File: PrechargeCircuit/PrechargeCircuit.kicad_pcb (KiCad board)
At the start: 2 copper layers, 102.6 x 57.8 mm, 53 parts, among them J1 430450428, J2 430450428, J4 436500228, U1 TEA 1-0505E, U2 AMC1351DWVR, U3 AMC1351DWVR, U6 OP284EPZ

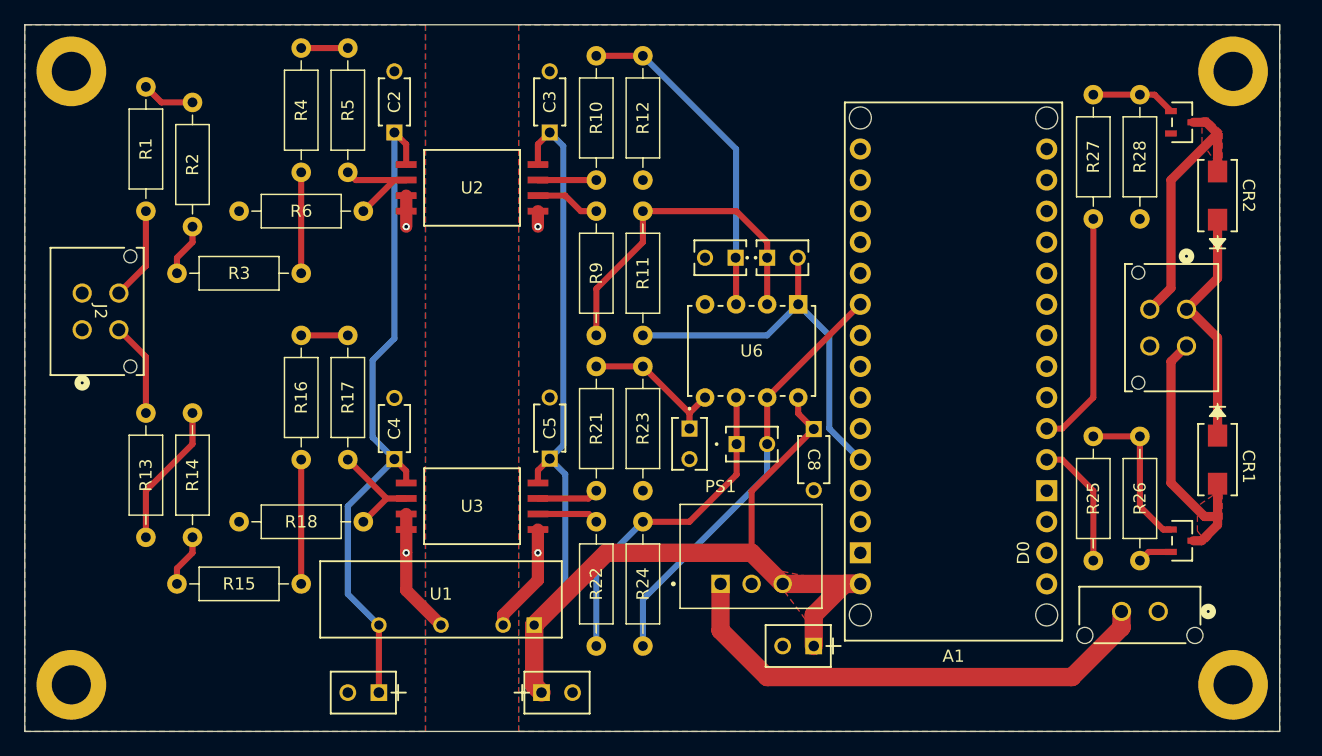
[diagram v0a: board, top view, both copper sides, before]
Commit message: V2
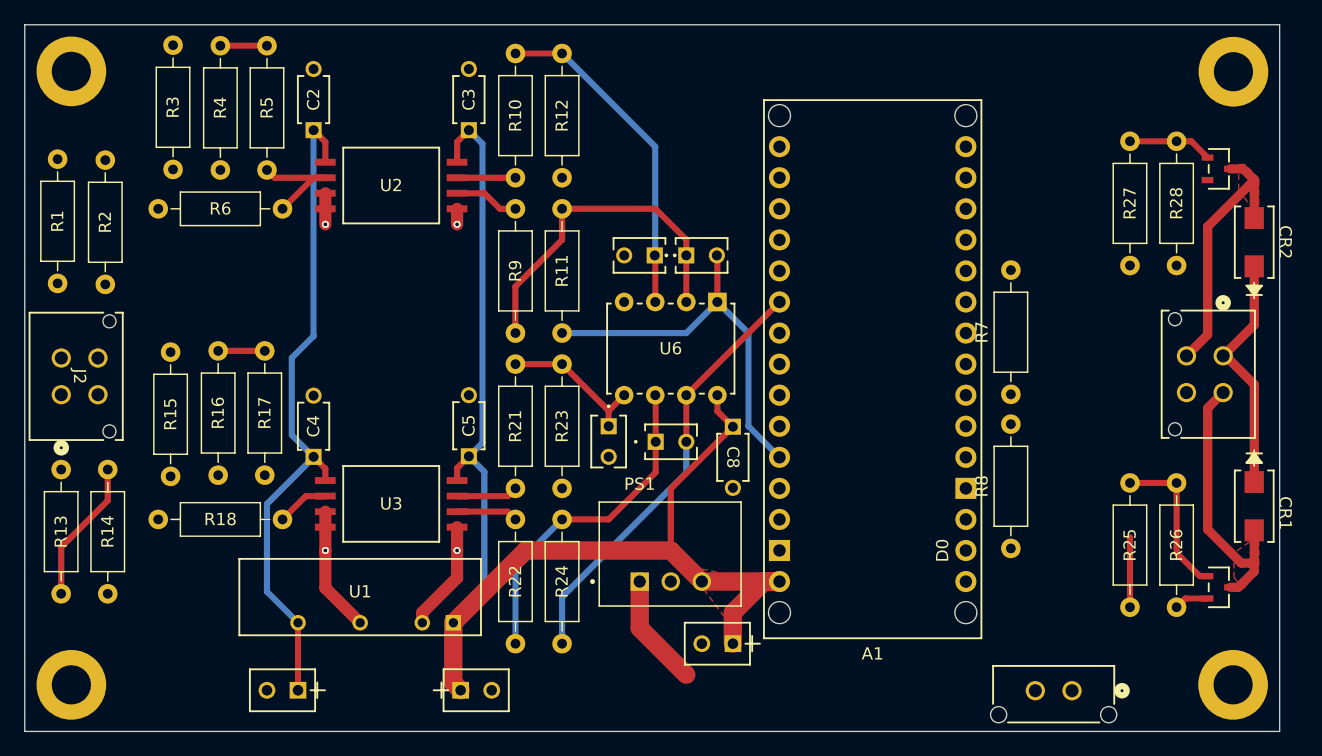
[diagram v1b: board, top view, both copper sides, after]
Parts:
- added R7: R_US, Resistor_THT:R_Axial_DIN0207_L6.3mm_D2.5mm_P10.16mm_Horizontal, F.Cu at (186.3, 91.2)
- added R8: R_US, Resistor_THT:R_Axial_DIN0207_L6.3mm_D2.5mm_P10.16mm_Horizontal, F.Cu at (186.3, 103.8)
- moved R15 19.0 mm to (117.6, 87.7), turned to -90 degrees
- moved R3 18.7 mm to (117.8, 62.6), turned to -90 degrees
- moved R2 16.5 mm to (112.2, 82.2), turned to 90 degrees
- moved J4 9.58 mm to (189.8, 115.7)
- moved R1 9.33 mm to (108.3, 82.1)
- moved R13 8.33 mm to (108.6, 97.3)
- moved R14 8.33 mm to (112.5, 97.3)
- moved R16 6.91 mm to (121.5, 97.8)
- moved R17 6.91 mm to (125.3, 87.6)
- moved A1 6.61 mm to (175.0, 67.1)
- moved C1 6.61 mm to (163.6, 111.6)
- moved C10 6.61 mm to (153.4, 93.8)
- moved C11 6.61 mm to (128.0, 115.4)
- moved C3 6.61 mm to (142.0, 69.6)
- moved C5 6.61 mm to (142.0, 96.2)
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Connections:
- A1 pad D4: unconnected-(A1-PadD4) -> /SenseSHD
- J2 pad 2: /HVGND -> /InverterGND
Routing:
- net Net-(PS1-+VIN): track 41.2 -> 9.20 mm
- net Net-(A1-PadD3): track 19.5 -> 0.00 mm
- net Net-(R15-Pad2): track 10.2 -> 0.00 mm
- net Net-(R3-Pad2): track 8.25 -> 0.00 mm
- net Net-(J2-Pad3): track 7.73 -> 0.00 mm
- net Net-(J2-Pad4): track 7.62 -> 0.00 mm
- net Net-(A1-PadD2): track 10.6 -> 5.72 mm
- net Net-(U3-IN): track 8.78 -> 4.29 mm
- net Net-(R14-Pad2): track 4.34 -> 0.00 mm
- net Net-(R2-Pad2): track 4.34 -> 0.00 mm
- net Net-(R1-Pad2): track 4.34 -> 0.00 mm
- removed copper zone on B.Cu, net /HVGND
- removed copper zone on F.Cu, net /HVGND
- removed copper zone on B.Cu, net GND
- removed copper zone on F.Cu, net GND
